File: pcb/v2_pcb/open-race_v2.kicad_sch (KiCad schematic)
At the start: 0 parts

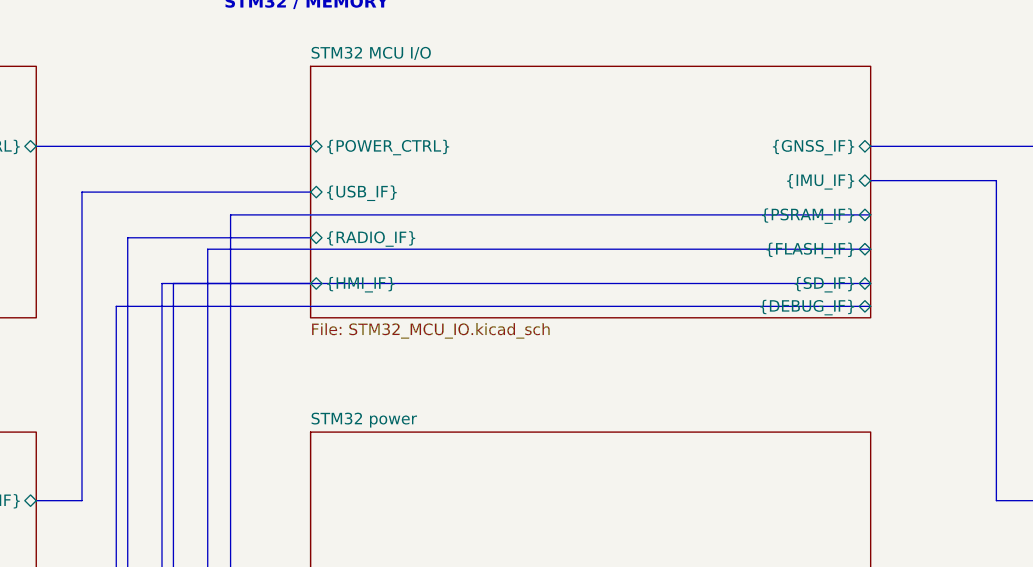
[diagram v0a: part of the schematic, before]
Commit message: power and debug cleanup
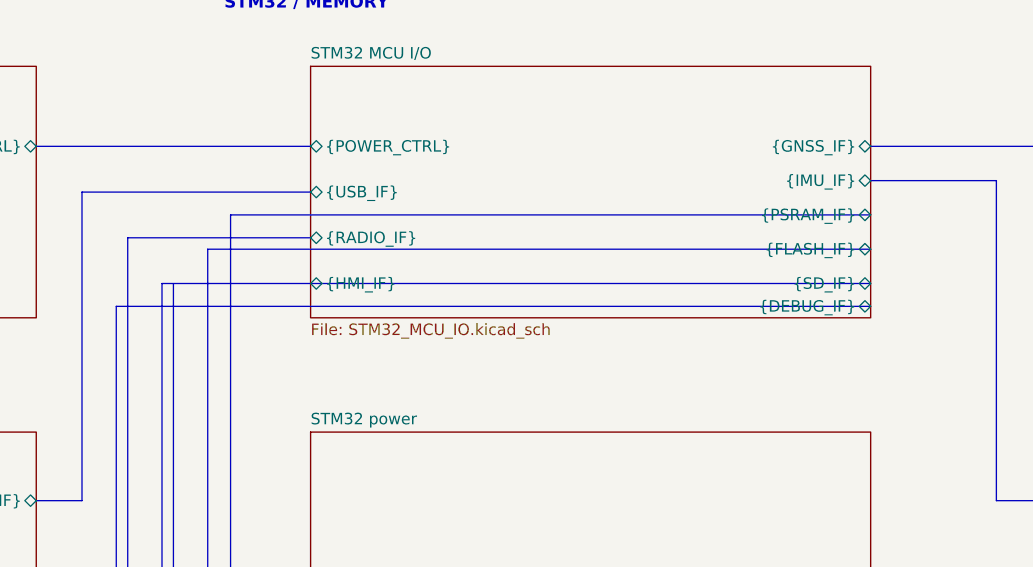
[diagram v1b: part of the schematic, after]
